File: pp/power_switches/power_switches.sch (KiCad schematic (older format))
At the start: 8 parts, among them J1 Screw_Terminal_1x02, J2 Screw_Terminal_1x02, P1 CONN_01X02, U1 MOC3063M

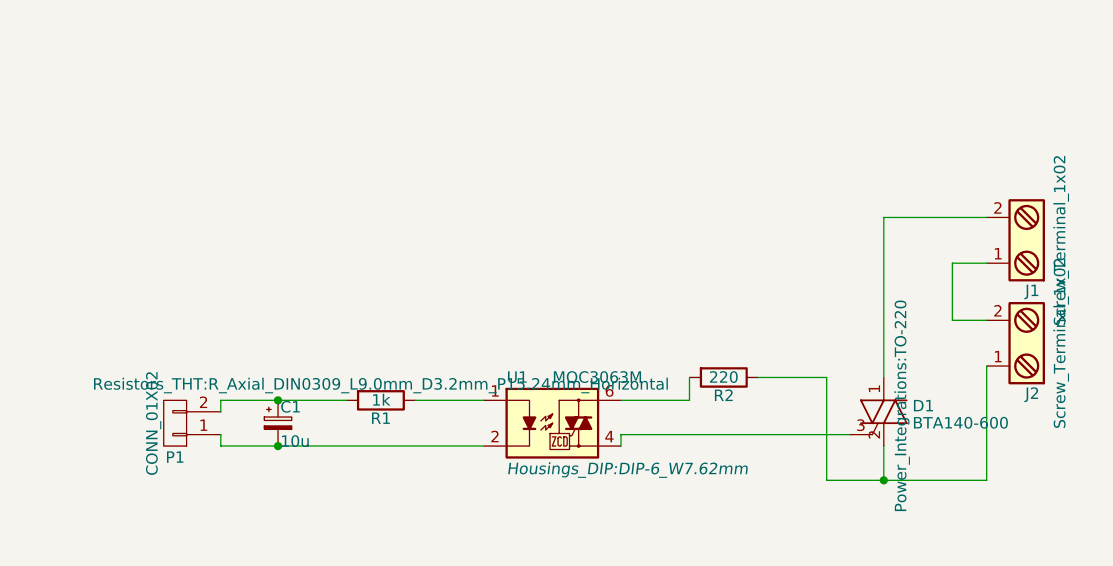
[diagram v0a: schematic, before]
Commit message: силовые ключи
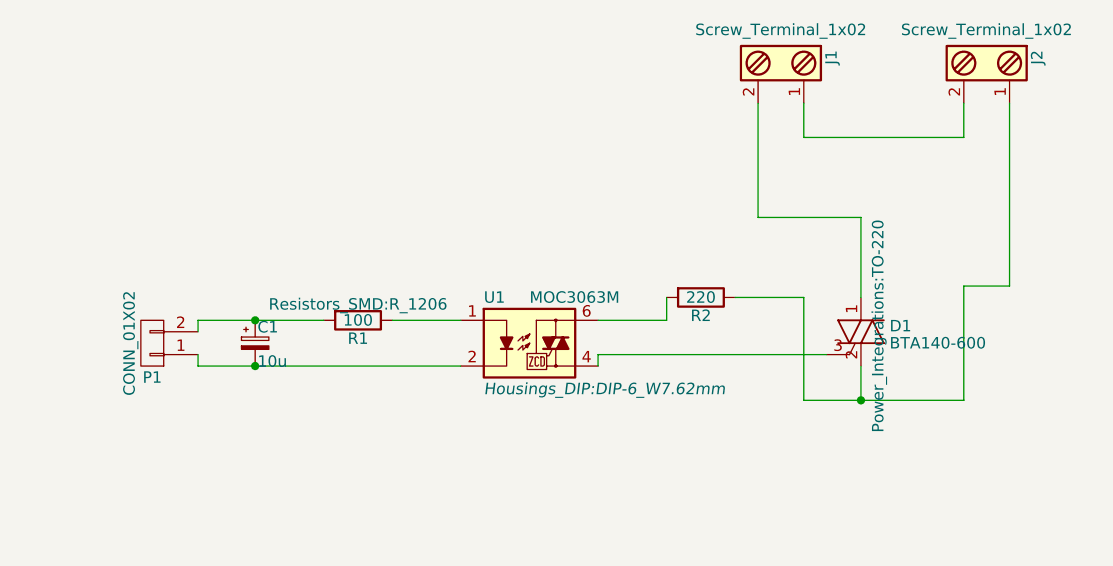
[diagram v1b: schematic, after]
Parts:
- J1, J2: footprint Connectors:AK300-2 -> Connectors_Terminal_Blocks:TerminalBlock_Pheonix_MPT-2.54mm_2pol
- P1: footprint Connectors_Terminal_Blocks:TerminalBlock_Pheonix_MPT-2.54mm_2pol -> Socket_Strips:Socket_Strip_Straight_1x02_Pitch2.54mm
- R1: value 1k -> 100; footprint Resistors_THT:R_Axial_DIN0309_L9.0mm_D3.2mm_P15.24mm_Horizontal -> Resistors_SMD:R_1206
- R2: footprint Resistors_THT:R_Axial_DIN0309_L9.0mm_D3.2mm_P15.24mm_Horizontal -> Resistors_SMD:R_1206
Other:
- moved on the sheet: C1, D1, J1, J2, P1, R1, R2, U1
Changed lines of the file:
@@
 L MOC3063M U1
 U 1 1 596A6E9F
-P 3900 3900
-F 0 "U1" H 3700 4100 50  0000 L CNN
-F 1 "MOC3063M" H 3900 4100 50  0000 L CNN
-F 2 "Housings_DIP:DIP-6_W7.62mm" H 3700 3700 50  0000 L CIN
-F 3 "" H 3890 3900 50  0000 L CNN
-	1    3900 3900
+P 3800 3550
+F 0 "U1" H 3600 3750 50  0000 L CNN
+F 1 "MOC3063M" H 3800 3750 50  0000 L CNN
+F 2 "Housings_DIP:DIP-6_W7.62mm" H 3600 3350 50  0000 L CIN
+F 3 "" H 3790 3550 50  0000 L CNN
+	1    3800 3550
 	1    0    0    -1
 $EndComp
@@
 L R R2
 U 1 1 596A7123
-P 4650 3700
-F 0 "R2" V 4730 3700 50  0000 C CNN
-F 1 "220" V 4650 3700 50  0000 C CNN
-F 2 "Resistors_THT:R_Axial_DIN0309_L9.0mm_D3.2mm_P15.24mm_Horizontal" V 4580 3700 50  0001 C CNN
-F 3 "" H 4650 3700 50  0000 C CNN
-	1    4650 3700
+P 4550 3350
+F 0 "R2" V 4630 3350 50  0000 C CNN
+F 1 "220" V 4550 3350 50  0000 C CNN
+F 2 "Resistors_SMD:R_1206" V 4480 3350 50  0001 C CNN
+F 3 "" H 4550 3350 50  0000 C CNN
+	1    4550 3350
 	0    1    1    0
 $EndComp
 Wire Wire Line
-	5200 3950 4200 3950
+	5100 3600 4100 3600
 Wire Wire Line
-	4200 3950 4200 4000
+	4100 3600 4100 3650
 Wire Wire Line
-	4800 3700 5100 3700
+	4700 3350 5000 3350
 Wire Wire Line
-	5100 3700 5100 4150
+	5000 3350 5000 3800
 Wire Wire Line
-	5100 4150 5800 4150
+	5000 3800 5700 3800
 Wire Wire Line
-	5350 4150 5350 4000
+	5250 3800 5250 3650
 Wire Wire Line
-	4200 3800 4500 3800
+	4100 3450 4400 3450
 Wire Wire Line
-	4500 3800 4500 3700
+	4400 3450 4400 3350
 $Comp
 L R R1
 U 1 1 596A71C3
-P 3150 3800
-F 0 "R1" V 3230 3800 50  0000 C CNN
-F 1 "1k" V 3150 3800 50  0000 C CNN
-F 2 "Resistors_THT:R_Axial_DIN0309_L9.0mm_D3.2mm_P15.24mm_Horizontal" V 3080 3800 50  0000 C CNN
-F 3 "" H 3150 3800 50  0000 C CNN
-	1    3150 3800
+P 3050 3450
+F 0 "R1" V 3130 3450 50  0000 C CNN
+F 1 "100" V 3050 3450 50  0000 C CNN
+F 2 "Resistors_SMD:R_1206" V 2980 3450 50  0000 C CNN
+F 3 "" H 3050 3450 50  0000 C CNN
+	1    3050 3450
 	0    1    1    0
 $EndComp
 Wire Wire Line
-	3600 3800 3300 3800
+	3500 3450 3200 3450
 $Comp
 L CP_Small C1
 U 1 1 596A7243
-P 2700 3900
-F 0 "C1" H 2710 3970 50  0000 L CNN
-F 1 "10u" H 2710 3820 50  0000 L CNN
-F 2 "Capacitors_THT:CP_Radial_D5.0mm_P2.50mm" H 2700 3900 50  0001 C CNN
-F 3 "" H 2700 3900 50  0000 C CNN
-	1    2700 3900
+P 2600 3550
+F 0 "C1" H 2610 3620 50  0000 L CNN
+F 1 "10u" H 2610 3470 50  0000 L CNN
+F 2 "Capacitors_THT:CP_Radial_D5.0mm_P2.50mm" H 2600 3550 50  0001 C CNN
+F 3 "" H 2600 3550 50  0000 C CNN
+	1    2600 3550
 	1    0    0    -1
 $EndComp
 Wire Wire Line
-	2450 3800 3000 3800
+	2350 3450 2900 3450
 Wire Wire Line
-	2450 4000 3600 4000
+	2350 3650 3500 3650
 $Comp
 L Screw_Terminal_1x02 J1
 U 1 1 596A72C0
-P 6000 3100
-F 0 "J1" H 6000 3350 50  0000 C TNN
-F 1 "Screw_Terminal_1x02" V 5850 3100 50  0000 C TNN
-F 2 "Connectors:AK300-2" H 6000 2875 50  0001 C CNN
-F 3 "" H 5975 3100 50  0001 C CNN
-	1    6000 3100
-	-1   0    0    1
+P 4900 2300
+F 0 "J1" H 4900 2550 50  0000 C TNN
+F 1 "Screw_Terminal_1x02" V 4750 2300 50  0000 C TNN
+F 2 "Connectors_Terminal_Blocks:TerminalBlock_Pheonix_MPT-2.54mm_2pol" H 4900 2075 50  0001 C CNN
+F 3 "" H 4875 2300 50  0001 C CNN
+	1    4900 2300
+	0    1    1    0
 $EndComp
 $Comp
 L Screw_Terminal_1x02 J2
 U 1 1 596A735F
-P 6000 3550
-F 0 "J2" H 6000 3800 50  0000 C TNN
-F 1 "Screw_Terminal_1x02" V 5850 3550 50  0000 C TNN
-F 2 "Connectors:AK300-2" H 6000 3325 50  0001 C CNN
-F 3 "" H 5975 3550 50  0001 C CNN
-	1    6000 3550
-	-1   0    0    1
+P 5800 2300
+F 0 "J2" H 5800 2550 50  0000 C TNN
+F 1 "Screw_Terminal_1x02" V 5650 2300 50  0000 C TNN
+F 2 "Connectors_Terminal_Blocks:TerminalBlock_Pheonix_MPT-2.54mm_2pol" H 5800 2075 50  0001 C CNN
+F 3 "" H 5775 2300 50  0001 C CNN
+	1    5800 2300
+	0    1    1    0
 $EndComp
 Wire Wire Line
-	5800 3200 5650 3200
-Wire Wire Line
-	5650 3200 5650 3450
-Wire Wire Line
-	5650 3450 5800 3450
-Wire Wire Line
-	5800 3000 5350 3000
-Wire Wire Line
-	5350 3000 5350 3700
-Wire Wire Line
-	5800 4150 5800 3650
-Connection ~ 5350 4150
+	5700 3800 5700 3300
+Connection ~ 5250 3800
 $Comp
 L BTA140-600 D1
 U 1 1 596A7C62
-P 5350 3850
-F 0 "D1" H 5475 3875 50  0000 L CNN
-F 1 "BTA140-600" H 5475 3800 50  0000 L CNN
-F 2 "Power_Integrations:TO-220" V 5425 3875 50  0000 C CNN
-F 3 "" V 5350 3850 50  0000 C CNN
-	1    5350 3850
+P 5250 3500
+F 0 "D1" H 5375 3525 50  0000 L CNN
+F 1 "BTA140-600" H 5375 3450 50  0000 L CNN
+F 2 "Power_Integrations:TO-220" V 5325 3525 50  0000 C CNN
+F 3 "" V 5250 3500 50  0000 C CNN
+	1    5250 3500
 	1    0    0    -1
 $EndComp
@@
 L CONN_01X02 P1
 U 1 1 596A835D
-P 2250 3900
-F 0 "P1" H 2250 4050 50  0000 C CNN
-F 1 "CONN_01X02" V 2350 3900 50  0000 C CNN
-F 2 "Connectors_Terminal_Blocks:TerminalBlock_Pheonix_MPT-2.54mm_2pol" H 2250 3900 50  0001 C CNN
-F 3 "" H 2250 3900 50  0000 C CNN
-	1    2250 3900
+P 2150 3550
+F 0 "P1" H 2150 3700 50  0000 C CNN
+F 1 "CONN_01X02" V 2250 3550 50  0000 C CNN
+F 2 "Socket_Strips:Socket_Strip_Straight_1x02_Pitch2.54mm" H 2150 3550 50  0001 C CNN
+F 3 "" H 2150 3550 50  0000 C CNN
+	1    2150 3550
 	-1   0    0    1
 $EndComp
 Wire Wire Line
-	2450 3800 2450 3850
-Connection ~ 2700 3800
+	2350 3450 2350 3500
+Connection ~ 2600 3450
 Wire Wire Line
-	2450 4000 2450 3950
-Connection ~ 2700 4000
+	2350 3650 2350 3600
+Connection ~ 2600 3650
+Wire Wire Line
+	5000 2500 5000 2650
+Wire Wire Line
+	5000 2650 5700 2650
+Wire Wire Line
+	5700 2650 5700 2500
+Wire Wire Line
+	5250 3350 5250 3000
+Wire Wire Line
+	5250 3000 4800 3000
+Wire Wire Line
+	4800 3000 4800 2500
+Wire Wire Line
+	5700 3300 5900 3300
+Wire Wire Line
+	5900 3300 5900 2500
 $EndSCHEMATC
